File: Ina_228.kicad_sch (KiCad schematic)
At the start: 13 parts, among them U1 INA228AQDGSRQ1

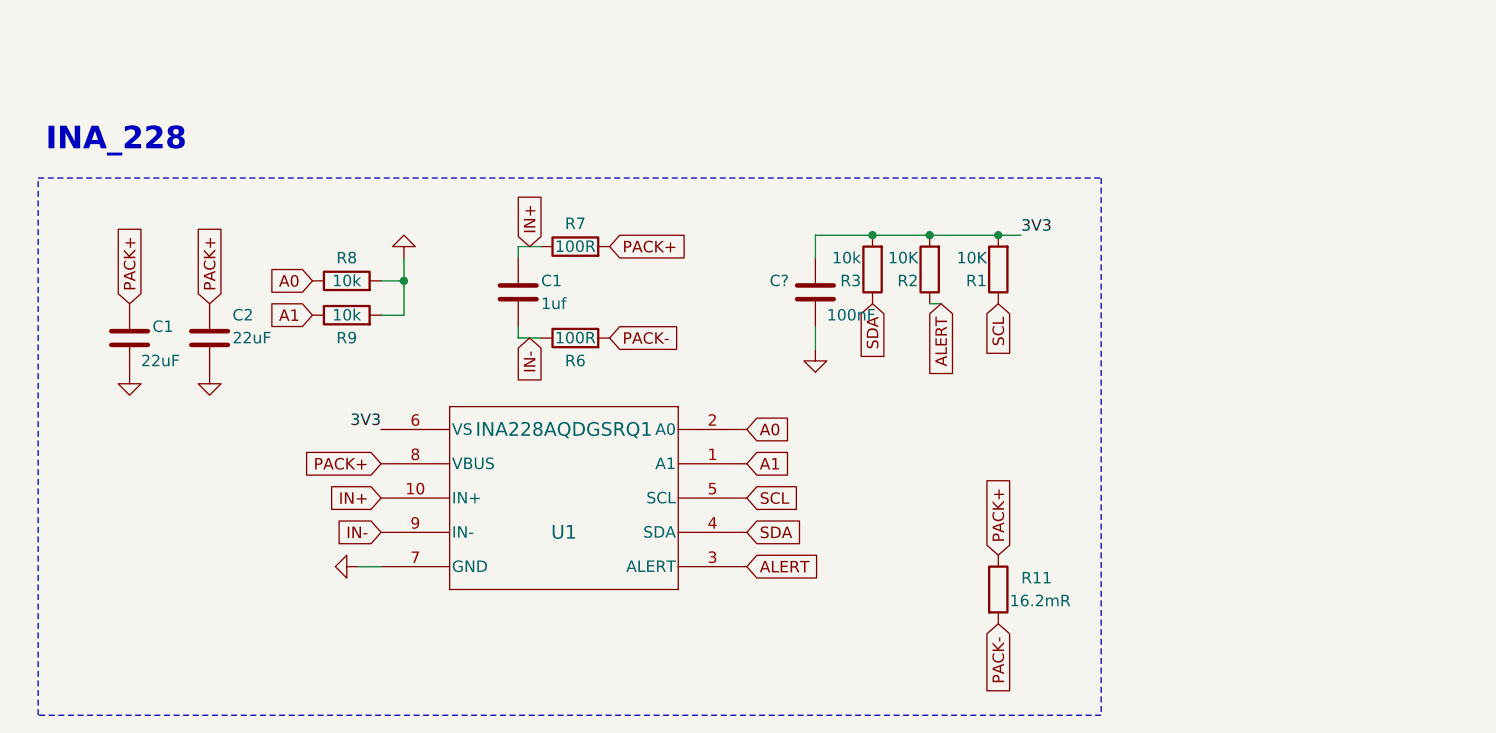
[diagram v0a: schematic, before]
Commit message: NAYE
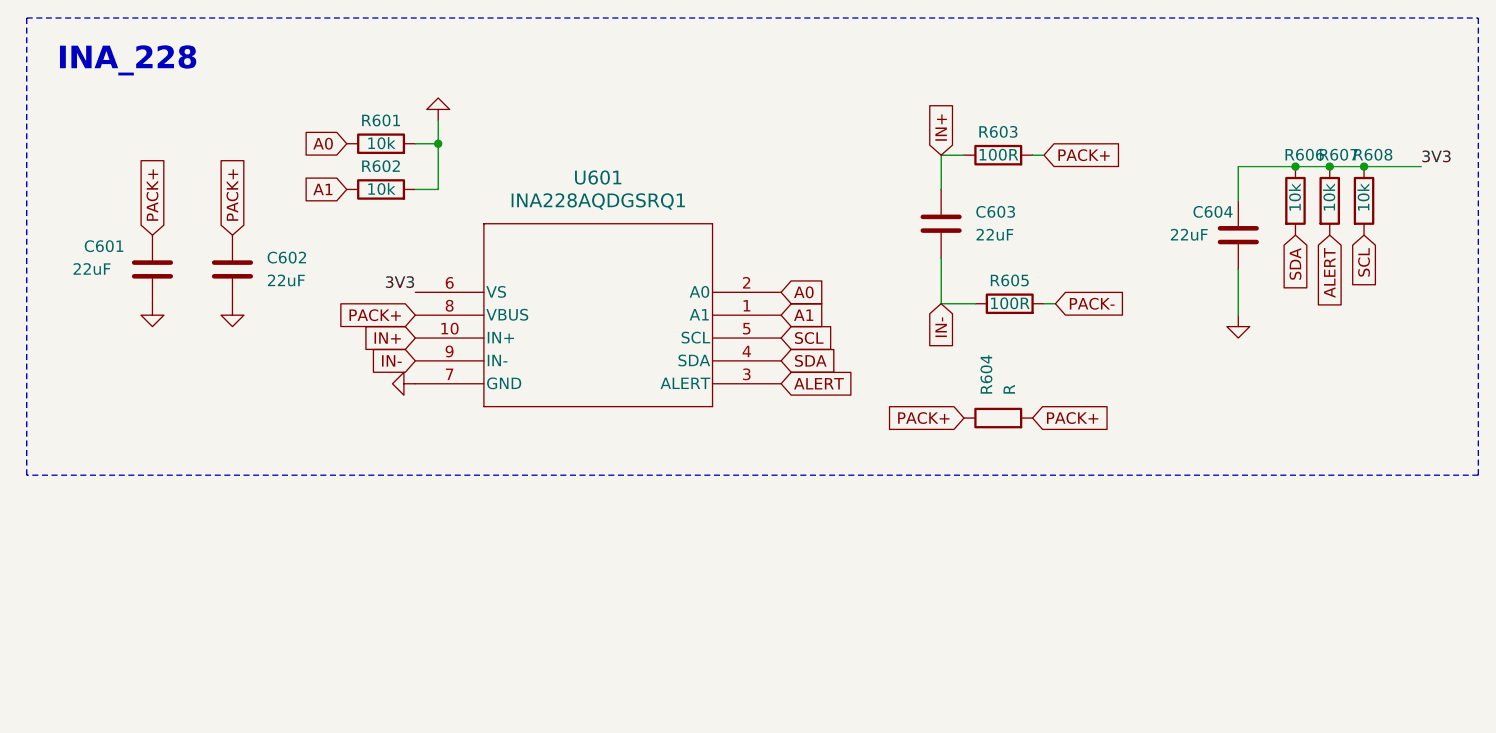
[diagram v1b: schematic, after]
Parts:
- removed C1, C2: 22uF, symbol Device:C
- removed C1: 1uf, symbol Device:C
- removed C?: 100nF, symbol Device:C
- removed R1, R2: 10K, symbol Device:R
- removed R11: 16.2mR, symbol Device:R
- removed R3, R8, R9: 10k, symbol Device:R
- removed R6, R7: 100R, symbol Device:R
- removed U1: INA228AQDGSRQ1, VSSOP10_DGS_TEX, symbol INA:INA228AQDGSRQ1
- added C601, C602, C603, C604: 22uF, symbol Device:C
- added R601, R602, R606, R607, R608: 10k, symbol Device:R
- added R603, R605: 100R, symbol Device:R
- added R604: R, symbol Device:R
- added U601: INA228AQDGSRQ1, VSSOP10_DGS_TEX, symbol 2023-08-04_10-34-25:INA228AQDGSRQ1
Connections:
- net 3V3: now also C604.1, R606.1, R607.1, R608.1, U601.6 (VS)
- net A0: now also R601.1, U601.2 (A0)
- net A1: now also R602.1, U601.1 (A1)
- net ALERT: now also R607.2, U601.3 (ALERT)
- net GND: now also C601.2, C602.2, C604.2, R601.2, R602.2, U601.7 (GND)
- net IN+: now also C603.1, R603.1, U601.10 (IN+)
- net IN-: now also C603.2, R605.1, U601.9 (IN-)
- net PACK+: now also C601.1, C602.1, R603.2, R604.1, R604.2, U601.8 (VBUS)
- net PACK-: now also R605.2
- net SCL: now also R608.2, U601.5 (SCL)
- net SDA: now also R606.2, U601.4 (SDA)
